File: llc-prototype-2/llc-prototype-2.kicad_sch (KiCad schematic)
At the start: 10 parts, among them J1 HV+, J2 HV-, T1 Transformer_1P_SS, U1 UCC256612DDBR, U2 UCC24624DR

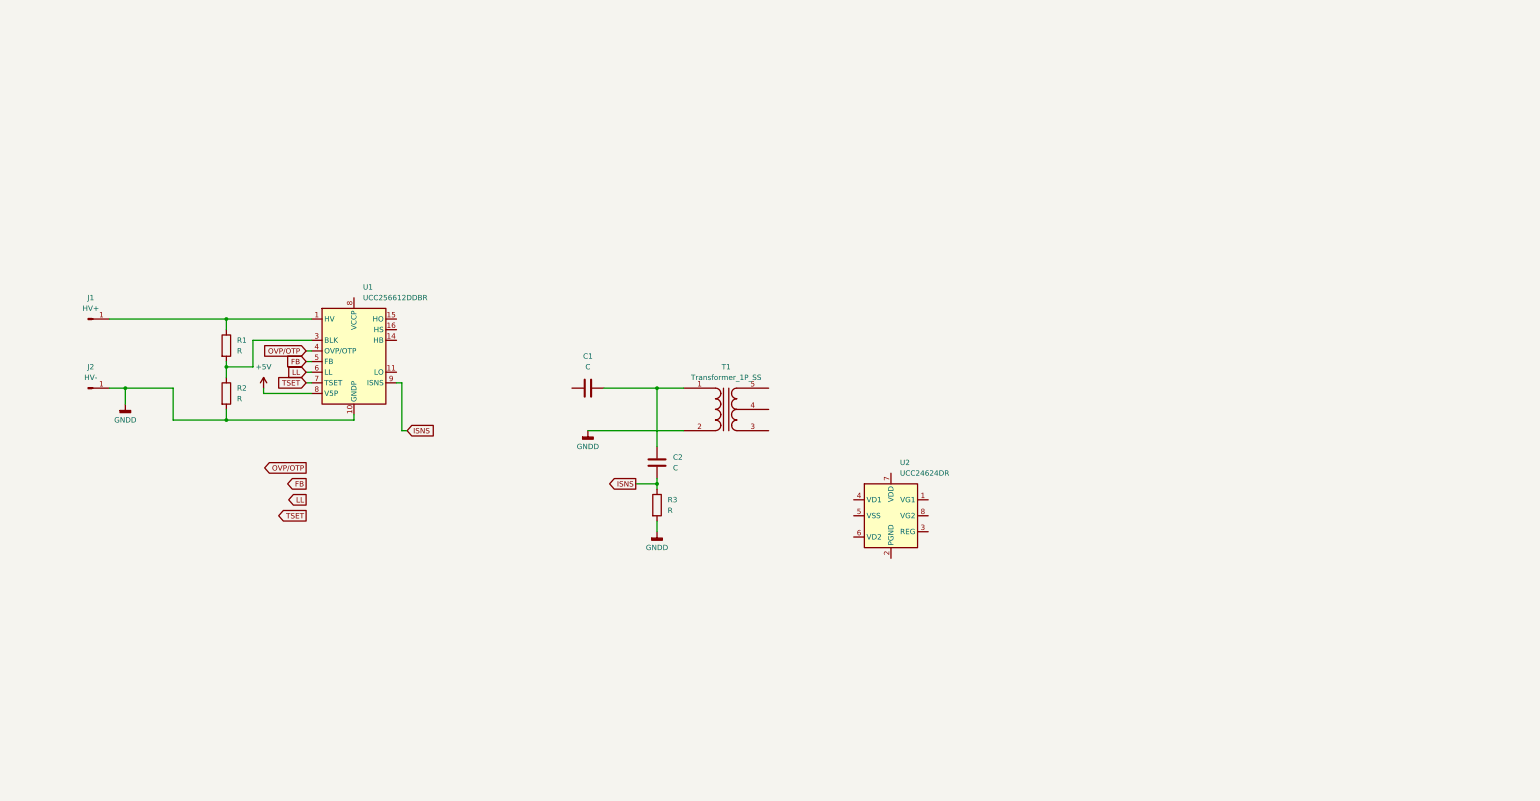
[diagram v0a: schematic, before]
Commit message: Rev 1.1
Finished Power Stage
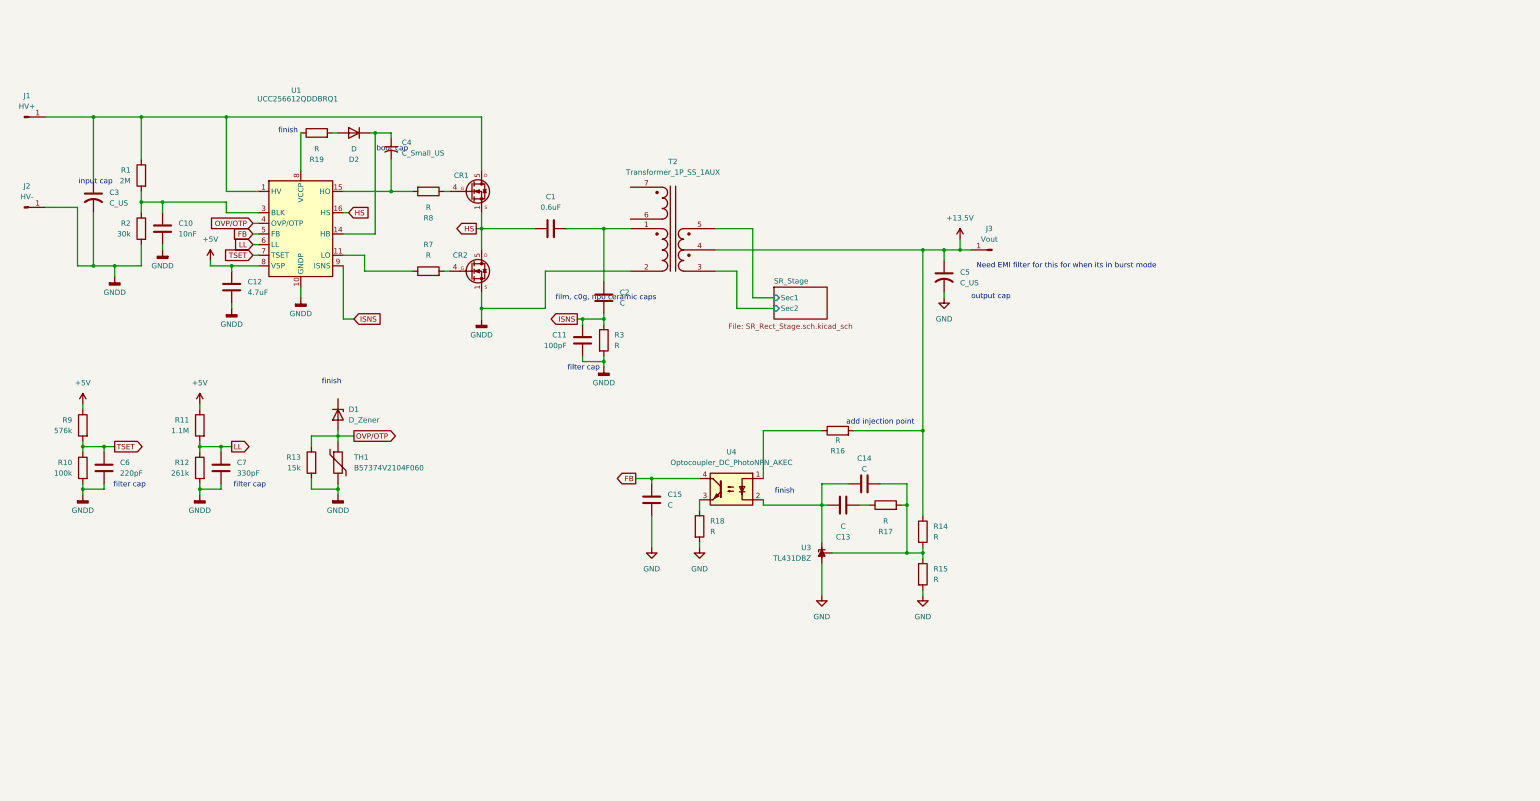
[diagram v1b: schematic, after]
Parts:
- removed T1: Transformer_1P_SS, symbol Device:Transformer_1P_SS
- removed U2: UCC24624DR, Package_SO:SOIC-8-1EP_3.9x4.9mm_P1.27mm_EP2.29x3mm_ThermalVias, symbol formula_slug_symbol_library:UCC24624DR
- added C10: 10nF, symbol Device:C
- added C11: 100pF, symbol Device:C
- added C12: 4.7uF, symbol Device:C
- added C13, C14, C15: C, symbol Device:C
- added C3, C5: C_US, symbol Device:C_US
- added C4: C_Small_US, symbol Device:C_Small_US
- added C6: 220pF, symbol Device:C
- added C7: 330pF, symbol Device:C
- added CR1, CR2: (no value), formula_slug_footprint_library:SO-8_STM, symbol formula_slug_symbol_library:STS6NF20V
- added D1: D_Zener, symbol Device:D_Zener
- added D2: D, symbol Device:D
- added J3: Vout, symbol Connector:Conn_01x01_Pin
- added R10: 100k, symbol Device:R
- added R11: 1.1M, symbol Device:R
- added R12: 261k, symbol Device:R
- added R13: 15k, symbol Device:R
- added R14, R15, R16, R17, R18, R19, R7, R8: R, symbol Device:R
- added R9: 576k, symbol Device:R
- added T2: Transformer_1P_SS_1AUX, symbol formula_slug_symbol_library:Transformer_1P_SS_1AUX
- added TH1: B57374V2104F060, symbol Device:Thermistor
- added U3: TL431DBZ, Package_TO_SOT_SMD:SOT-23, symbol Reference_Voltage:TL431DBZ
- added U4: Optocoupler_DC_PhotoNPN_AKEC, symbol Isolator:Optocoupler_DC_PhotoNPN_AKEC
- C1: value C -> 0.6uF
- R1: value R -> 2M
- R2: value R -> 30k
- U1: value UCC256612DDBR -> UCC256612QDDBRQ1
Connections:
- net +5V: now also C12.2, R11.1, R9.1
- net FB: now also C15.1, U4.4
- net GNDD: now also C10.1, C11.1, C12.1, C3.2, C6.1, C7.1, CR2.1 (S), CR2.2 (S), CR2.3 (S), R10.2, R12.2, R13.2, T2.2 (AB), TH1.2
- net ISNS: now also C11.2
- net LL: now also C7.2, R11.2, R12.1
- net OVP/OTP: now also D1.2 (A), R13.1, TH1.1
- net TSET: now also C6.2, R10.1, R9.2
- net at R1.2, R2.1, U1.3 (BLK): now also C10.2
- net at J1.1 (Pin_1), R1.1, U1.1 (HV): now also C3.1, CR1.5 (D), CR1.6 (D), CR1.7 (D), CR1.8 (D)
- net at U1.11 (LO): now also R7.1
- net at U1.14 (HB): now also C4.1, D2.1 (K)
- net at U1.15 (HO): now also C4.2, R8.2
- net HS: now reaches U1.16 (HS)
- net HS: now also C1.1, CR1.1 (S), CR1.2 (S), CR1.3 (S), CR2.5 (D), CR2.6 (D), CR2.7 (D), CR2.8 (D)
- net at C1.2, C2.2: now also T2.1 (AA)
- new net: R16.1, U4.1
- new net: C13.1, C14.1, U3.1 (K), U4.2
- new net: R18.1, U4.3
- new net: R19.1, U1.8 (VCCP)
- new net: D2.2 (A), R19.2
- new net: C14.2, R14.2, R15.1, R17.2, U3.2 (REF)
- new net: CR1.4 (G), R8.1
- new net: CR2.4 (G), R7.2
- new net: C13.2, R17.1
- new net +13.5V: C5.1, J3.1 (Pin_1), R14.1, R16.2, T2.4 (SC)
- new net GND: C15.2, C5.2, R15.2, R18.2, U3.3 (A)
- new net SR_Stage/Sec1: T2.5 (SB)
- new net SR_Stage/Sec2: T2.3 (SA)
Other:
- added sheet SR_Stage (SR_Rect_Stage.sch.kicad_sch)
- note added: "Need EMI filter for this for when its in burst mode"
- note added: "add injection point"
- note added: "boot cap"
- note added: "film, c0g, np0 ceramic caps"
- note added: "filter cap"
- note added: "finish"
- note added: "input cap"
- note added: "output cap"
- moved on the sheet: C1, C2, J1, J2, R1, R2, R3, U1

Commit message: Rev 1.2
added output caps, resonant caps, feedback compensation, fast turn off for primary fets
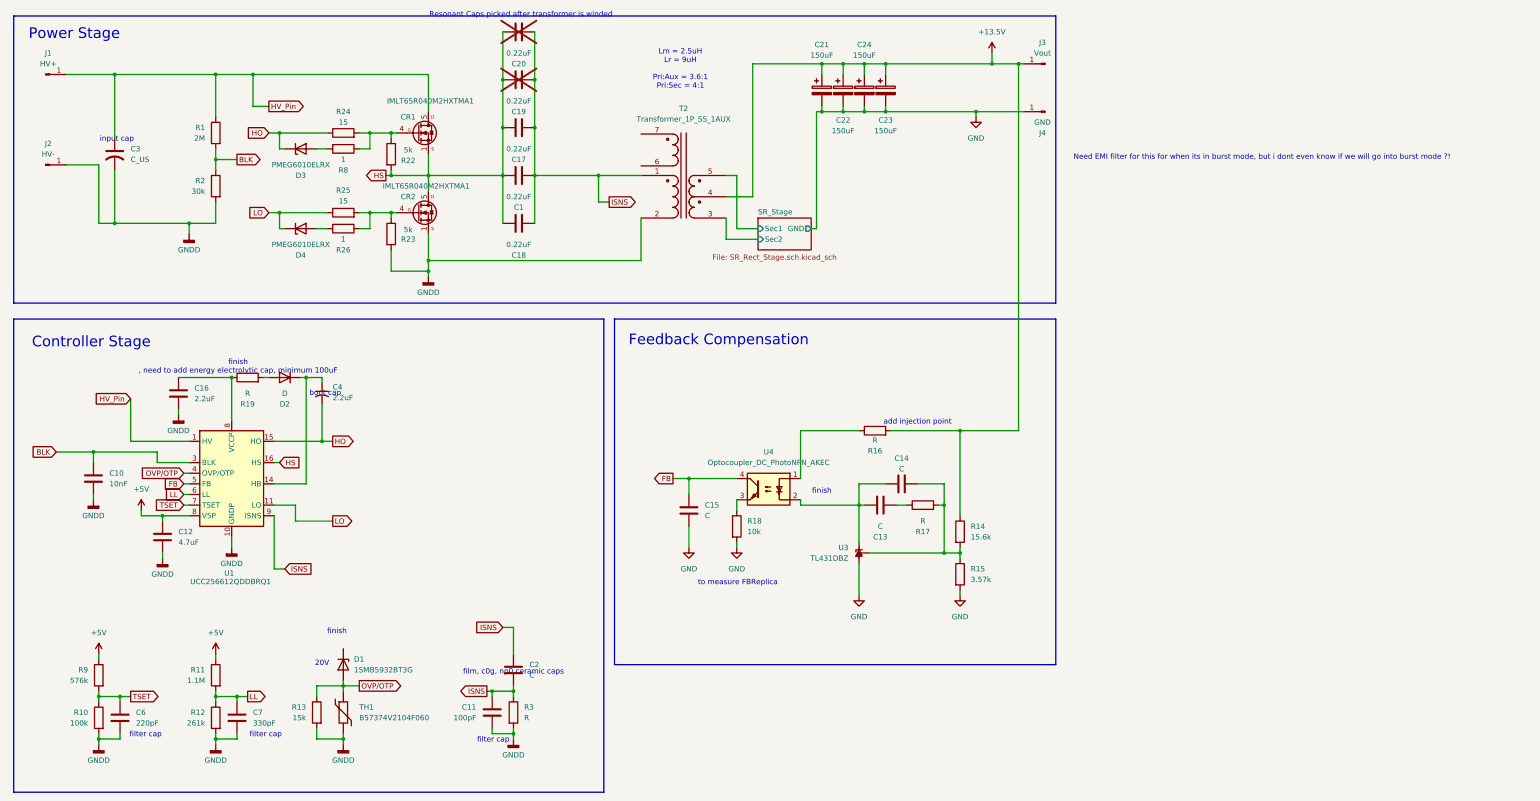
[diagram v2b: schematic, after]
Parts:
- removed C5: C_US, symbol Device:C_US
- removed R7: R, symbol Device:R
- added C16: 2.2uF, symbol Device:C
- added C17, C18, C19, C20: 0.22uF, symbol Device:C
- added C21, C22, C23, C24: 150uF, symbol Device:C_Polarized
- added D3, D4: PMEG6010ELRX, symbol Device:D_Zener
- added J4: GND, symbol Connector:Conn_01x01_Pin
- added R22, R23: 5k, symbol Device:R
- added R24, R25: 15, symbol Device:R
- added R26: 1, symbol Device:R
- C1: value 0.6uF -> 0.22uF
- C4: value C_Small_US -> 2.2uF
- CR1, CR2: value (none) -> IMLT65R040M2HXTMA1; Digikey Part Number (none) -> 448-IMLT65R040M2HXTMA1CT-ND; Digikey URL (none) -> https://www.digikey.com/en/products/detail/infineon-technol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; Manufacturer (none) -> Infineon Technologies; Manufacturer Part Number (none) -> IMLT65R040M2HXTMA1
- D1: value D_Zener -> 1SMB5932BT3G; Digikey URL (none) -> https://www.digikey.com/en/products/detail/onsemi/1SMB5932B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
- R14: value R -> 15.6k
- R15: value R -> 3.57k
- R18: value R -> 10k
- R8: value R -> 1
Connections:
- net +13.5V: now also C21.1, C22.1, C23.1, C24.1
- net GND: now also C21.2, C22.2, C23.2, C24.2, J4.1 (Pin_1)
- net GNDD: now also C16.1, R23.2
- net HS: now also C17.1, C18.1, C19.1, C20.1, R22.2
- net ISNS: now also C1.2, C2.2, T2.1 (AA), C17.2, C18.2, C19.2, C20.2
- net HO: now reaches C4.2, U1.15 (HO)
- net HO: now also D3.1 (K), R24.1; no longer R8.2
- net BLK: now reaches C10.2, R1.2, R2.1, U1.3 (BLK)
- net at R19.1, U1.8 (VCCP): now also C16.2
- net at CR1.4 (G), R8.1: now also R22.1, R24.2
- net HV_Pin: now reaches C3.1, CR1.5 (D), CR1.6 (D), CR1.7 (D), CR1.8 (D), J1.1 (Pin_1), R1.1, U1.1 (HV)
- net LO: now reaches U1.11 (LO)
- net LO: now also D4.1 (K), R25.1
- net at CR2.4 (G): now also R23.1, R25.2, R26.1
- new net: D3.2 (A), R8.2
- new net: D4.2 (A), R26.2
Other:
- sheet SR_Stage ports: added GND; removed none
- note added: "20V"
- note added: "Controller Stage"
- note added: "Feedback Compensation"
- note added: "Lm = 2.5uH Lr = 9uH Pri:Aux = 3.6:1 Pri:Sec = 4:1"
- note added: "Need EMI filter for this for when its in burst mode, but i dont even know if we will go into burst mode ?!"
- note added: "Power Stage"
- note added: "Resonant Caps picked after transformer is winded"
- note added: "finish , need to add energy electrolytic cap, minimum 100uF"
- note added: "to measure FBReplica"
- note removed: "Need EMI filter for this for when its in burst mode"
- note removed: "output cap"
- moved on the sheet: C1, C10, C11, C12, C13, C14, C15, C2, C3, C4, C6, C7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
